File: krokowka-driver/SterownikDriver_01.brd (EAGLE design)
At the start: 60.6 x 45.7 mm, 56 parts, among them IC1 NC7WP14P6X, IC4 NC7WP14P6X, Q1 IRF3704S, Q2 IRF3704S, Q3 IRF3704S, Q4 IRF3704S, Q5 IRF3704S, Q6 IRF3704S, Q7 IRF3704S, Q8 IRF3704S, U1 IR2104, U2 IR2104, U3 IR2104, U4 IR2104

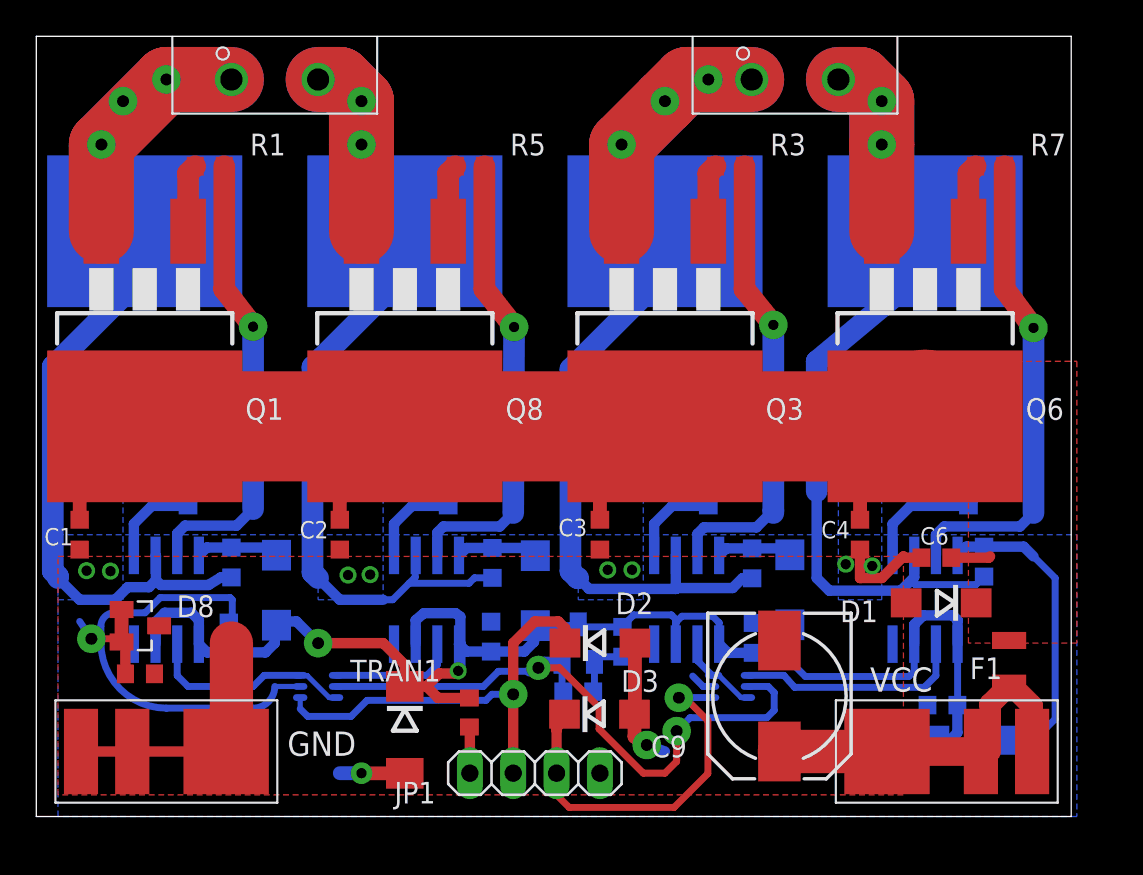
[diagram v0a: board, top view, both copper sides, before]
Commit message: ver 0.2
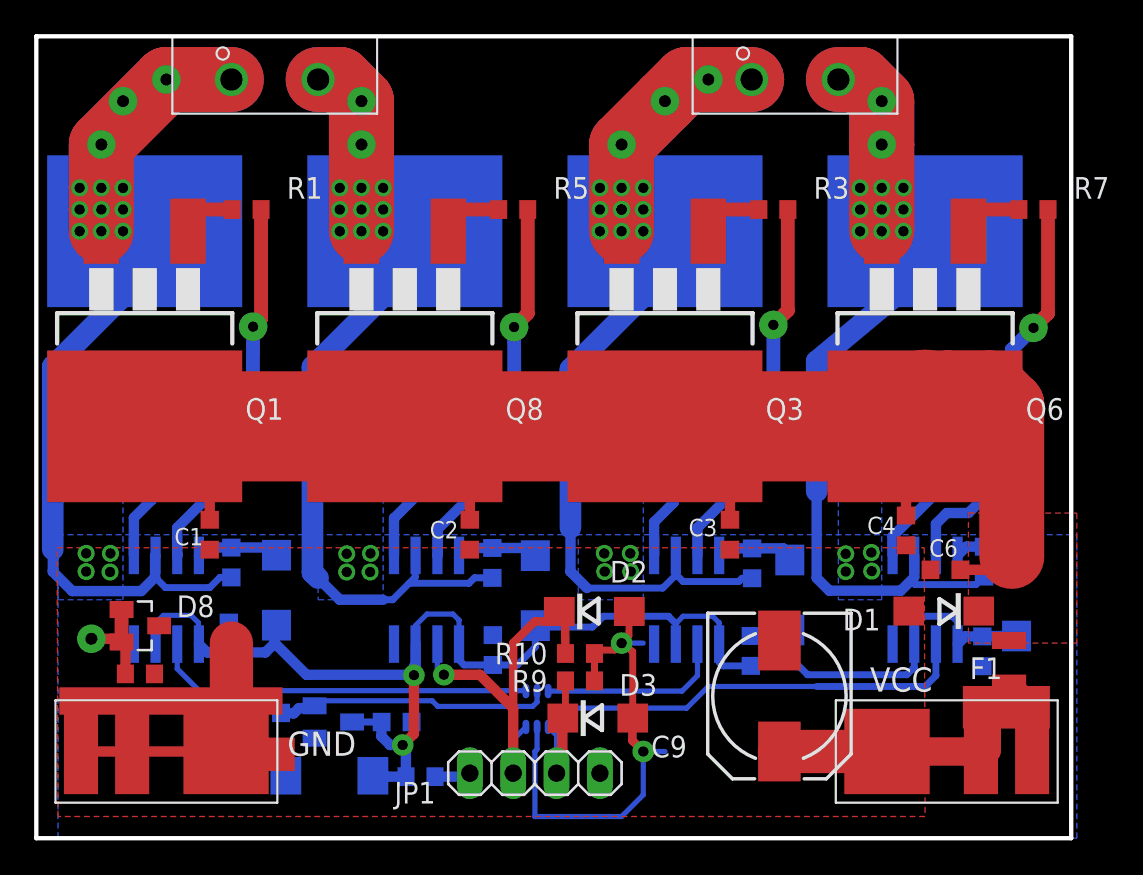
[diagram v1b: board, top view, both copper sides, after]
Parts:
- removed IC4: NC7WP14P6X, bufory,invertery:SOT65P210X110-6AN_SC88_SC70-6
- added R10, R9: 10, rcl:R0603
- moved C16 18.3 mm to (13.5, 6.07), turned to 0 degrees
- moved U$6 15.1 mm to (17.4, 5.54), turned to 90 degrees
- moved C17 14.0 mm to (21.1, 5.54), turned to 180 degrees
- moved IC1 12.9 mm to (29.3, 6.30), turned to 90 degrees
- moved D7 8.62 mm to (57.4, 12.6), turned to 270 degrees
- moved C1 7.62 mm to (10.2, 16.5)
- moved C2 7.62 mm to (25.4, 16.5)
- moved C3 7.62 mm to (40.6, 16.5)
- moved TRAN1 5.18 mm to (17.2, 2.39), flipped to the bottom, turned to 0 degrees
- moved U$3 4.73 mm to (22.5, 2.34), flipped to the bottom, turned to 0 degrees
- moved C14 3.92 mm to (55.4, 9.68), turned to 270 degrees
- moved R5 3.59 mm to (27.9, 35.6)
- moved R3 3.59 mm to (43.2, 35.6)
- moved R7 3.59 mm to (58.4, 35.6)
- moved R1 3.33 mm to (12.3, 35.6)
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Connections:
- removed net N$5: IC1.4, U2.2
- removed net N$6: IC4.4, U4.2
- net +3V3: no longer IC4.5
- net GND: now also R10.1, R9.1; no longer IC4.2
- net PWM1: now also IC1.3, R10.2, U2.2; no longer IC1.1
- net PWM1_NEG: now also IC1.4; no longer IC1.3, IC1.6
- net PWM2: now also IC1.1, R9.2, U4.2; no longer IC4.1
- net PWM2_NEG: now also IC1.6; no longer IC4.3, IC4.6
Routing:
- net +24V: track 76.4 -> 101.5 mm
- net +3V3: track 38.6 -> 16.2 mm, vias 2 -> 0
- net N$18: track 18.6 -> 4.69 mm
- net N$6: track 13.5 -> 0.00 mm, vias 0 -> 1
- net GND: track 48.3 -> 36.2 mm
- net PWM1_NEG: track 12.2 -> 22.5 mm
- net PWM2: track 24.9 -> 35.0 mm, vias 1 -> 0
- net N$5: track 7.40 -> 0.00 mm, vias 0 -> 1
- net PWM2_NEG: track 4.82 -> 11.0 mm
- net GNDA: track 20.2 -> 14.4 mm, vias 8 -> 16
- net N$14: track 27.2 -> 22.5 mm
- net N$7: track 27.2 -> 22.5 mm
- net N$3: track 27.0 -> 22.3 mm
- net N$20: track 28.3 -> 23.7 mm
- net PWM1: track 26.1 -> 23.5 mm
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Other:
- board size 60.6 x 45.7 mm -> 60.6 x 47 mm
- board text removed: "Czy tych złącz nie da się ścisnąć?"
